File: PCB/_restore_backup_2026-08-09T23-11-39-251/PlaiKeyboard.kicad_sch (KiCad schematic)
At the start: 177 parts, among them SW1 SW_Push_45deg, SW10 SW_Push_45deg, SW11 SW_Push_45deg, SW12 SW_Push_45deg, SW13 SW_Push_45deg, SW14 SW_Push_45deg, SW15 RotaryEncoder_Switch, SW16 SW_Push_45deg, SW17 SW_Push_45deg, SW18 SW_Push_45deg, SW19 SW_Push_45deg, SW2 SW_Push_45deg, SW20 SW_Push_45deg, SW21 SW_Push_45deg, SW22 SW_Push_45deg, SW23 SW_Push_45deg, SW24 SW_Push_45deg, SW25 SW_Push_45deg, SW26 SW_Push_45deg, SW27 SW_Push_45deg, SW28 SW_Push_45deg, SW29 SW_Push_45deg, SW3 SW_Push_45deg, SW30 SW_Push_45deg, SW31 SW_Push_45deg, SW32 SW_Push_45deg, SW33 SW_Push_45deg, SW34 SW_Push_45deg, SW35 SW_Push_45deg, SW36 SW_Push_45deg, SW37 SW_Push_45deg, SW38 SW_Push_45deg, SW39 SW_Push_45deg, SW4 SW_Push_45deg, SW40 SW_Push_45deg, SW41 SW_Push_45deg, SW42 SW_Push_45deg, SW43 SW_Push_45deg, SW44 SW_Push_45deg, SW45 SW_Push_45deg, SW46 SW_Push_45deg, SW47 SW_Push_45deg, SW48 SW_Push_45deg, SW49 SW_Push_45deg, SW5 SW_Push_45deg, SW50 SW_Push_45deg, SW51 SW_Push_45deg, SW52 SW_Push_45deg, SW53 SW_Push_45deg, SW54 SW_Push_45deg, SW55 SW_Push_45deg, SW56 SW_Push_45deg, SW57 SW_Push_45deg, SW58 SW_Push_45deg, SW59 SW_Push_45deg, SW6 SW_Push_45deg, SW60 SW_Push_45deg, SW61 SW_Push_45deg, SW62 SW_Push_45deg, SW63 SW_Push_45deg, SW64 SW_Push_45deg, SW65 SW_Push_45deg, SW66 SW_Push_45deg, SW67 SW_Push_45deg, SW68 SW_Push_45deg, SW69 SW_Push_45deg, SW7 SW_Push_45deg, SW70 SW_Push_45deg, SW71 SW_Push_45deg, SW72 SW_Push_45deg, SW73 SW_Push_45deg, SW74 SW_Push_45deg, SW75 SW_Push_45deg, SW76 SW_Push_45deg, SW77 SW_Push_45deg, SW78 SW_Push_45deg, SW79 SW_Push_45deg, SW8 SW_Push_45deg, SW80 SW_Push_45deg, SW81 SW_Push_45deg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

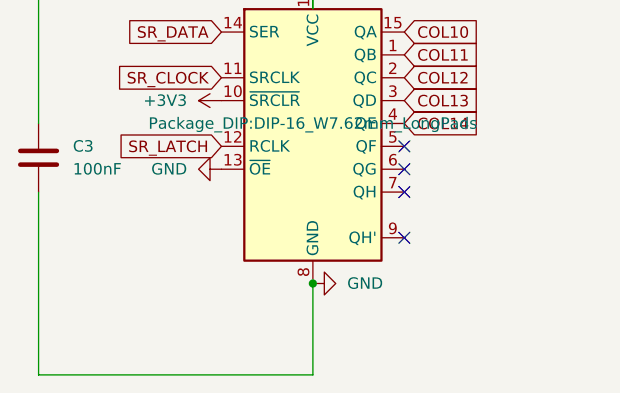
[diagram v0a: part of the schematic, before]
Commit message: ACTUALLY FINISHED WITH THE PCB
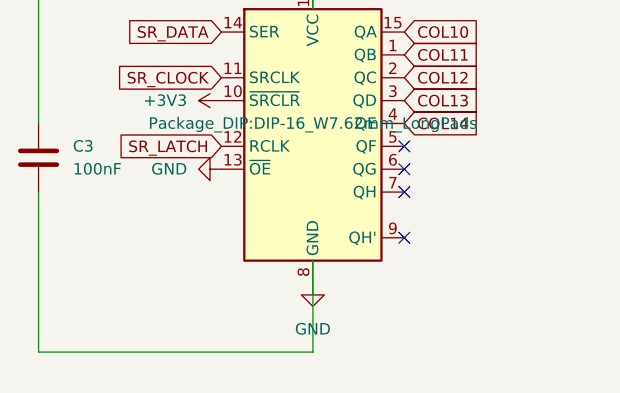
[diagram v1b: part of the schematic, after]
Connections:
- net GND: no longer C3.1
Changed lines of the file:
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@@
 	)
 	(junction
-		(at 57.15 287.02)
-		(diameter 0)
-		(color 0 0 0 0)
-	)
-	(junction
 		(at 236.22 165.1)
 		(diameter 0)
@@
 	(wire
 		(pts
-			(xy 26.67 297.18) (xy 26.67 276.86)
+			(xy 26.67 294.64) (xy 26.67 276.86)
 		)
 		(stroke
@@
 	(wire
 		(pts
-			(xy 26.67 297.18) (xy 57.15 297.18)
+			(xy 26.67 294.64) (xy 57.15 294.64)
 		)
 		(stroke
@@
 	(wire
 		(pts
-			(xy 57.15 297.18) (xy 57.15 287.02)
+			(xy 57.15 294.64) (xy 57.15 284.48)
 		)
 		(stroke
@@
 	(symbol
 		(lib_id "power:GND")
-		(at 57.15 287.02 90)
+		(at 57.15 287.02 0)
 		(unit 1)
 		(body_style 1)
@@
 		(fields_autoplaced yes)
 		(property "Reference" "#PWR013"
-			(at 63.5 287.02 0)
+			(at 57.15 293.37 0)
 			(hide yes)
 			(show_name no)
@@
 		)
 		(property "Value" "GND"
-			(at 60.96 287.0199 90)
+			(at 57.15 292.1 0)
 			(show_name no)
 			(do_not_autoplace no)
@@
 					(size 1.27 1.27)
 				)
-				(justify right)
 			)
 		)
